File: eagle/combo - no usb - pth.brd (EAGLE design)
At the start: 101.6 x 81.3 mm, 27 parts, among them U2 ATMEGA328P_PDIP

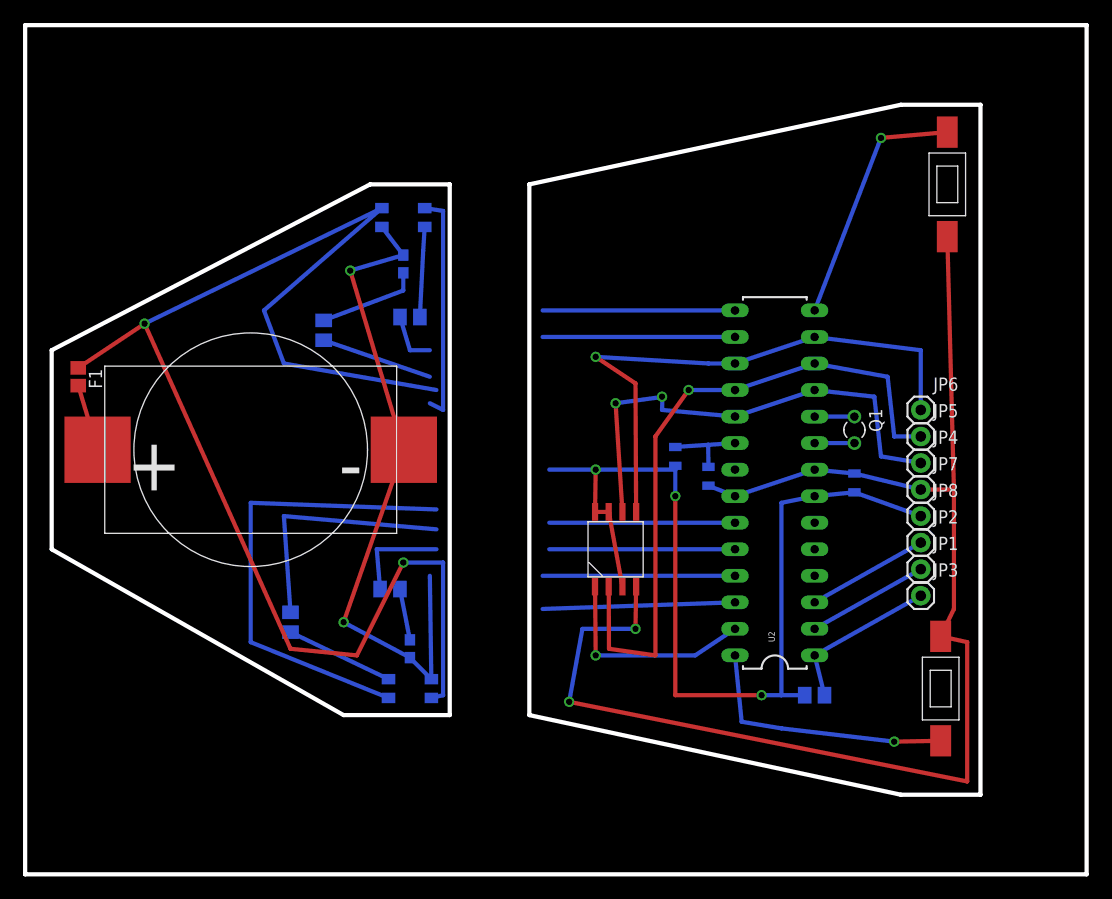
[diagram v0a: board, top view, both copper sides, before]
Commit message: Progress routing board
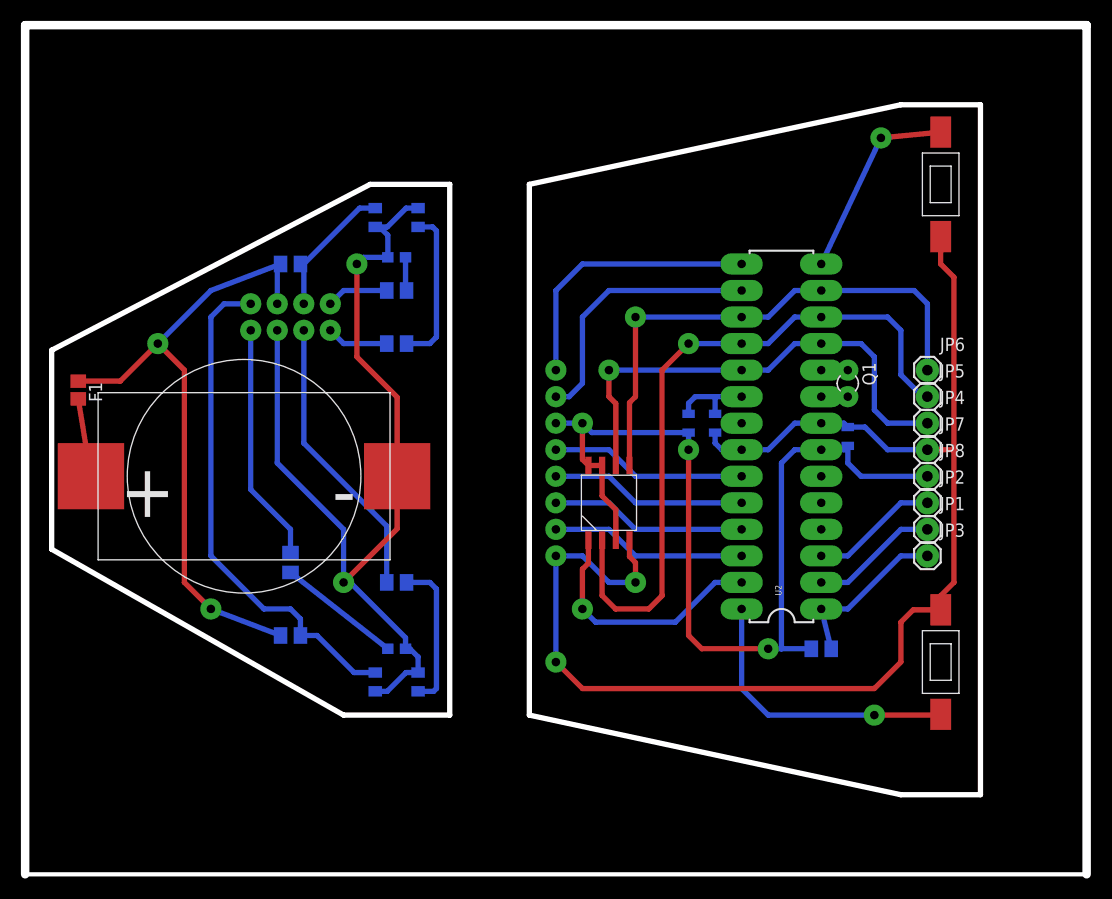
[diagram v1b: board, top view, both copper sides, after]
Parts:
- added R6, R7: (no value), rcl:M0805
- moved R2 10.9 mm to (35.6, 27.9), turned to 180 degrees
- moved R5 9.86 mm to (25.4, 29.8), turned to 270 degrees
- moved R4 7.96 mm to (35.6, 55.9), turned to 180 degrees
- moved C1 5.12 mm to (66.0, 43.2)
- moved U$8 4.49 mm to (55.9, 35.6)
- moved Q1 4.49 mm to (78.7, 47.0)
- moved R1 4.49 mm to (76.2, 21.6)
- moved C2 4.49 mm to (78.7, 41.9)
- moved U2 4.49 mm to (72.4, 41.9)
- moved JP1 3.86 mm to (86.4, 33.0)
- moved JP2 3.86 mm to (86.4, 35.6)
- moved JP4 3.86 mm to (86.4, 43.2)
- moved JP5 3.86 mm to (86.4, 45.7)
- moved JP7 3.86 mm to (86.4, 40.6)
- moved JP8 3.86 mm to (86.4, 38.1)
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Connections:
- net GND: now also U$3.EMITTER, U$4.EMITTER
- net IRSENS1: now also R7.1, U$3.COLLECTOR; no longer U$3.EMITTER
- net IRSENS2: now also R6.1, U$4.COLLECTOR; no longer U$4.EMITTER
- net VCC: now also R6.2, R7.2; no longer U$3.COLLECTOR, U$4.COLLECTOR
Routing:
- net VCC: track 227.8 -> 155.3 mm, vias 5 -> 7
- net GND: track 197.9 -> 221.6 mm, vias 4 -> 6
- net LED2: track 28.0 -> 48.6 mm, vias 0 -> 2
- net IRSENS2: track 40.0 -> 32.1 mm, vias 0 -> 2
- net N$13: track 4.96 -> 11.8 mm
- net N$15: track 8.64 -> 15.2 mm
- net N$14: track 9.83 -> 3.53 mm
- net BTN2: track 24.1 -> 19.1 mm
- net IRSENS1: track 63.1 -> 67.3 mm, vias 0 -> 2
- net N$16: track 10.4 -> 14.5 mm
- net IRLED1: track 42.3 -> 46.3 mm, vias 0 -> 2
- net MOSI: track 54.2 -> 50.3 mm
- net /CS: track 20.7 -> 24.2 mm
- net LED1: track 29.2 -> 32.4 mm, vias 0 -> 2
- net BTN1: track 25.6 -> 27.8 mm
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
